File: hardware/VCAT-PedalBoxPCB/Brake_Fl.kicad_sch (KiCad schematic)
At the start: 15 parts, among them U4 TLV70130DBVR, U5 AMC1300BDWV

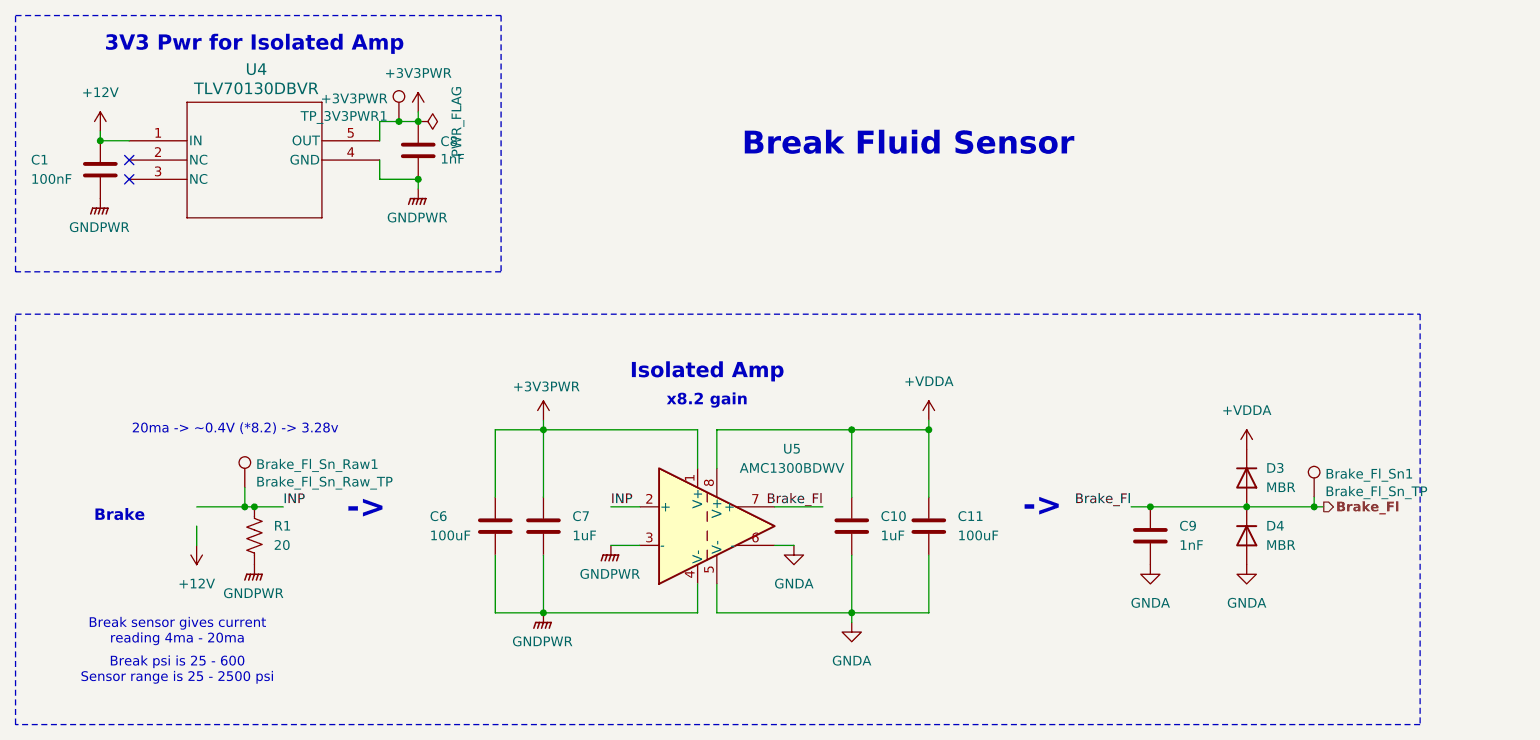
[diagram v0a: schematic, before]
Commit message: sch too ez
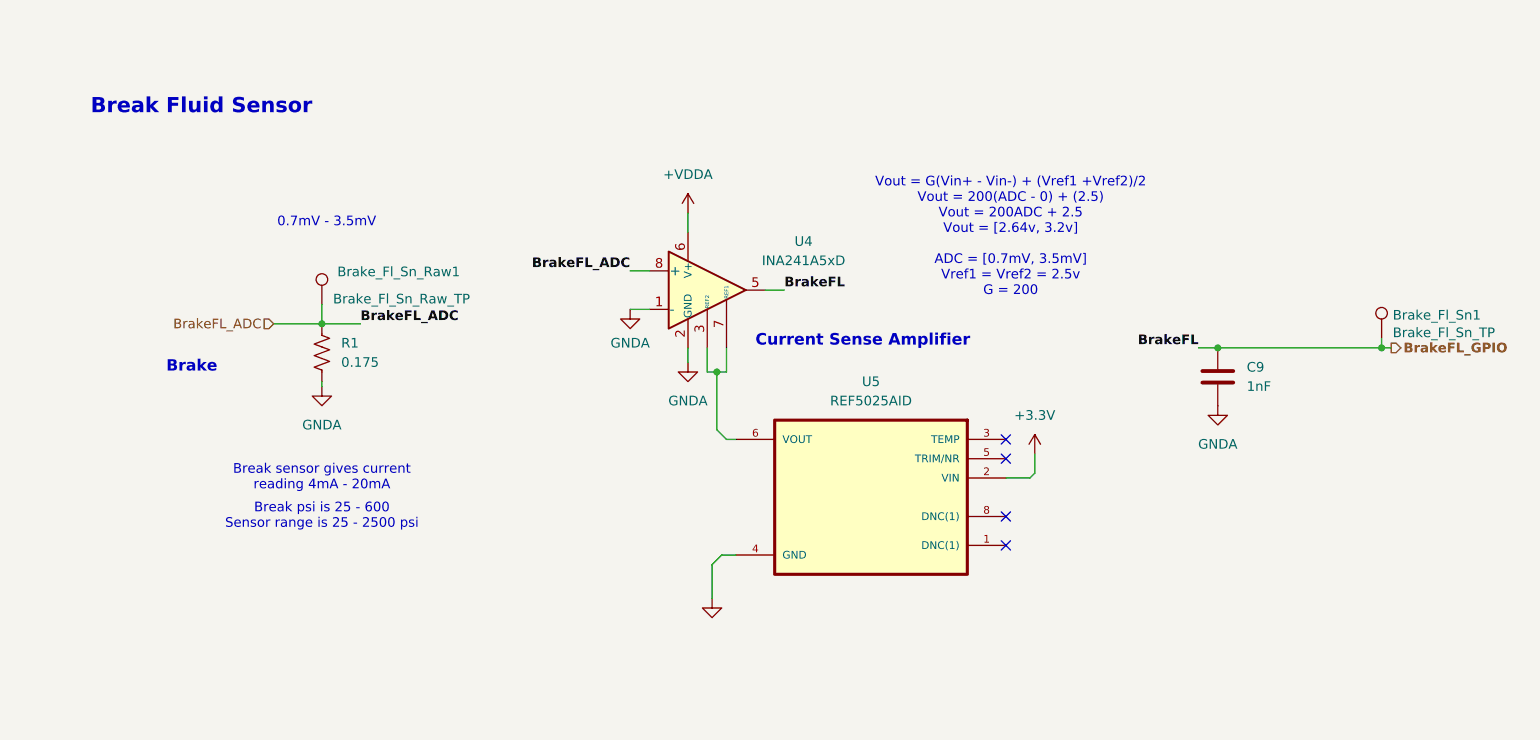
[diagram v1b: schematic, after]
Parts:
- removed C1: 100nF, Capacitor_SMD:C_0805_2012Metric, symbol Device:C
- removed C10, C7: 1uF, Capacitor_SMD:C_0805_2012Metric, symbol Device:C
- removed C11, C6: 100uF, Capacitor_SMD:C_0805_2012Metric, symbol Device:C
- removed C8: 1nF, Capacitor_SMD:C_0805_2012Metric, symbol Device:C
- removed D3, D4: MBR, Diode_SMD:D_0805_2012Metric, symbol Device:D
- removed TP_3V3PWR1: +3V3PWR, TestPoint:TestPoint_Pad_1.5x1.5mm, symbol Connector:TestPoint
- removed U4: TLV70130DBVR, Package_TO_SOT_SMD:SOT-353_SC-70-5, symbol 2025-01-18_20-51-31:TLV70130DBVR
- removed U5: AMC1300BDWV, Package_SO:SOIC-8_7.5x5.85mm_P1.27mm, symbol Amplifier_Difference:AMC1300BDWV
- added U4: INA241A5xD, Package_SO:SOIC-8_3.9x4.9mm_P1.27mm, symbol Amplifier_Current:INA241A5xD
- added U5: REF5025AID, REF5025AID:SOIC127P599X175-8N, symbol REF5025AID:REF5025AID
- R1: value 20 -> 0.175
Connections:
- net GNDPWR is gone; now on net GNDA: R1.2
- net +VDDA: now also U4.6 (V+)
- net GNDA: now also U4.1 (-), U4.2 (GND), U4.4 (GND)
- net Brake_Fl renamed BrakeFL_GPIO
- net BrakeFL_GPIO: now also U4.5
- net INP renamed BrakeFL_ADC
- net BrakeFL_ADC: now also U4.8 (+)
- new net: U4.3 (REF2), U4.7 (REF1), U5.6 (VOUT)
- new net +3.3V: U5.2 (VIN)
- new net GND: U5.4 (GND)
- no-connect marks 2 -> 4
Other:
- note added: "0.7mV - 3.5mV"
- note added: "Break sensor gives current reading 4mA - 20mA"
- note added: "Current Sense Amplifier"
- note added: "Vout = G(Vin+ - Vin-) + (Vref1 +Vref2)/2 Vout = 200(ADC - 0) + (2.5) Vout = 200ADC + 2.5 Vout = [2.64v, 3.2v] ADC = [0.7mV, 3.5mV] Vref1 = Vref2 = 2.5v G = 200"
- note removed: "->"
- note removed: "20ma -> ~0.4V (*8.2) -> 3.28v"
- note removed: "3V3 Pwr for Isolated Amp"
- note removed: "Break sensor gives current reading 4ma - 20ma"
- note removed: "Isolated Amp"
- note removed: "x8.2 gain"
- moved on the sheet: Brake_Fl_Sn1, Brake_Fl_Sn_Raw1, C9, R1
